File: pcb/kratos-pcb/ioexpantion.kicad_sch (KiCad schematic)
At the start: 3 parts, among them IC2 SN74HC595N, U3 ULN2803A

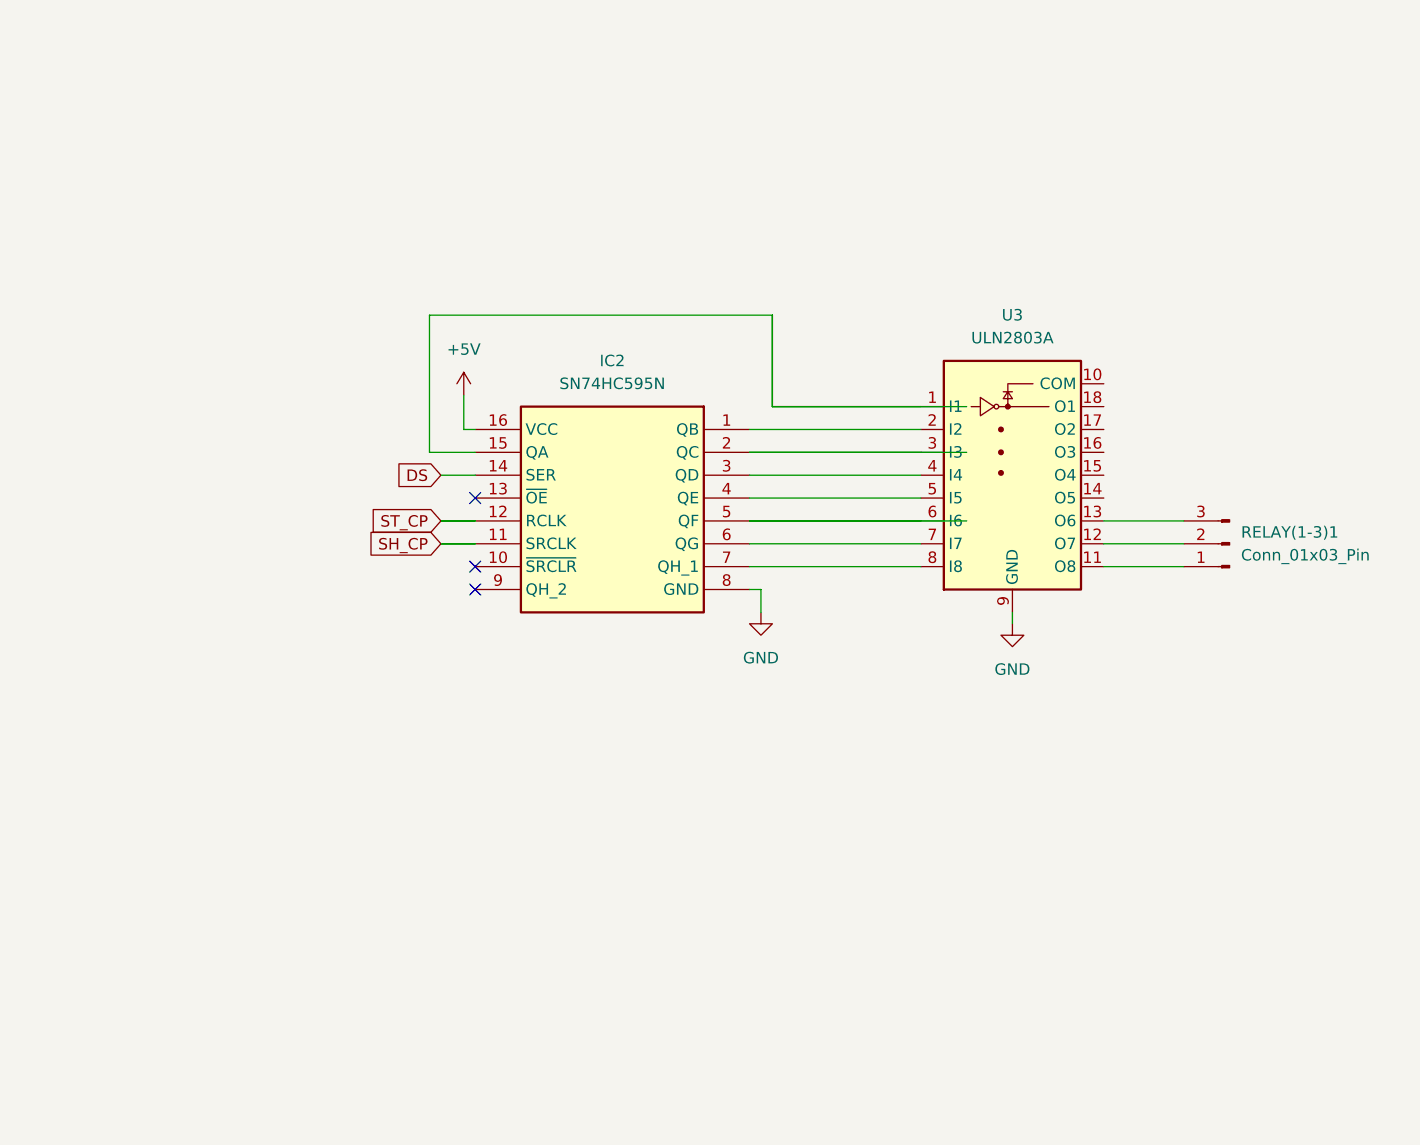
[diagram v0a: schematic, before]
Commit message: ### update     - kicad schematic
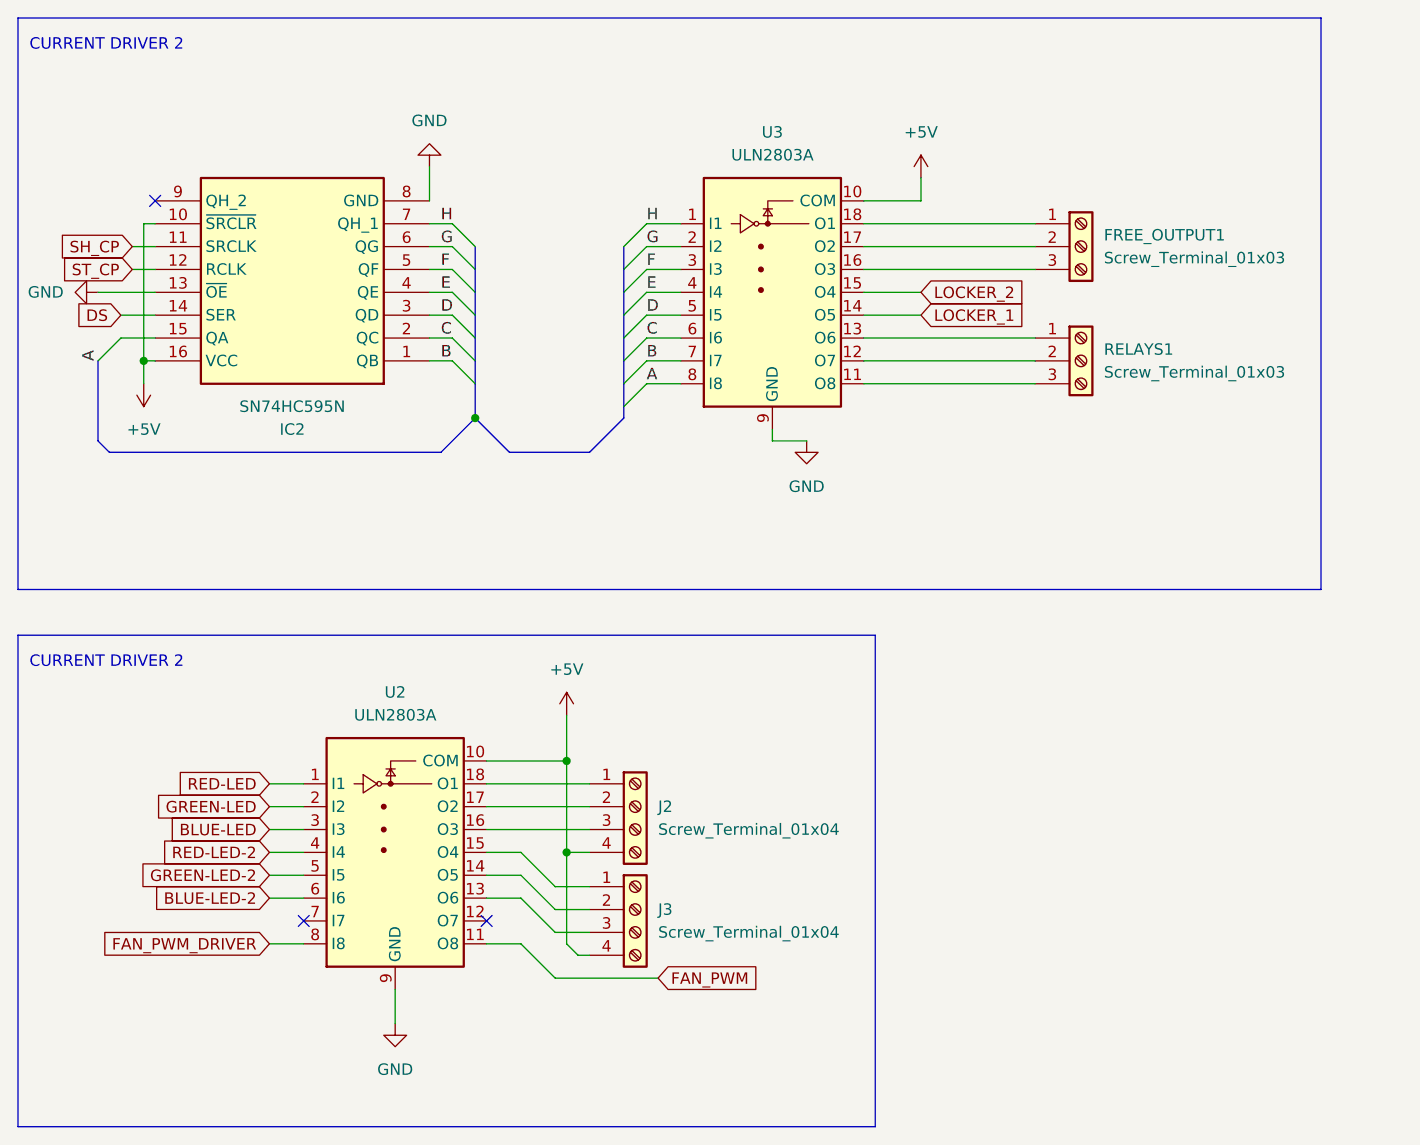
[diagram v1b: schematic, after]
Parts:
- removed RELAY(1-3)1: Conn_01x03_Pin, symbol Connector:Conn_01x03_Pin
- added FREE_OUTPUT1, RELAYS1: Screw_Terminal_01x03, TerminalBlock_4Ucon:TerminalBlock_4Ucon_1x03_P3.50mm_Horizontal, symbol Connector:Screw_Terminal_01x03
- added J2, J3: Screw_Terminal_01x04, TerminalBlock:TerminalBlock_bornier-4_P5.08mm, symbol Connector:Screw_Terminal_01x04
- added U2: ULN2803A, ULN2803A:ULN2803A, symbol Transistor_Array:ULN2803A
- IC2: footprint SN74HC595N:DIP794W53P254L1930H508Q16N -> DIP794W53P254L1930H508Q16N
- U3: footprint (none) -> ULN2803A:ULN2803A
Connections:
- net +5V: now also IC2.10 (~{SRCLR}), U3.10 (COM), J2.4 (Pin_4), J3.4 (Pin_4), U2.10 (COM)
- net GND: now also IC2.13 (~{OE}), U2.9 (GND)
- net B: now reaches IC2.1 (QB)
- net B: now also U3.7 (I7); no longer U3.2 (I2)
- net at IC2.15 (QA): no longer U3.1 (I1)
- net C: now reaches IC2.2 (QC)
- net C: now also U3.6 (I6); no longer U3.3 (I3)
- net D: now reaches IC2.3 (QD)
- net D: now also U3.5 (I5); no longer U3.4 (I4)
- net E: now reaches IC2.4 (QE)
- net E: now also U3.4 (I4); no longer U3.5 (I5)
- net F: now reaches IC2.5 (QF)
- net F: now also U3.3 (I3); no longer U3.6 (I6)
- net G: now reaches IC2.6 (QG)
- net G: now also U3.2 (I2); no longer U3.7 (I7)
- net A: now reaches U3.8 (I8)
- net A: no longer IC2.7 (QH_1)
- net at U3.11 (O8): now also RELAYS1.3 (Pin_3)
- net at U3.12 (O7): now also RELAYS1.2 (Pin_2)
- net at U3.13 (O6): now also RELAYS1.1 (Pin_1)
- net LOCKER_1: now reaches U3.14 (O5)
- net LOCKER_2: now reaches U3.15 (O4)
- net at U3.16 (O3): now also FREE_OUTPUT1.3 (Pin_3)
- net at U3.17 (O2): now also FREE_OUTPUT1.2 (Pin_2)
- net at U3.18 (O1): now also FREE_OUTPUT1.1 (Pin_1)
- new net: J3.3 (Pin_3), U2.13 (O6)
- new net: J3.2 (Pin_2), U2.14 (O5)
- new net: J3.1 (Pin_1), U2.15 (O4)
- new net: J2.3 (Pin_3), U2.16 (O3)
- new net: J2.2 (Pin_2), U2.17 (O2)
- new net: J2.1 (Pin_1), U2.18 (O1)
- new net BLUE-LED: U2.3 (I3)
- new net BLUE-LED-2: U2.6 (I6)
- new net FAN_PWM: U2.11 (O8)
- new net FAN_PWM_DRIVER: U2.8 (I8)
- new net GREEN-LED: U2.2 (I2)
- new net GREEN-LED-2: U2.5 (I5)
- new net H: IC2.7 (QH_1), U3.1 (I1)
- new net RED-LED: U2.1 (I1)
- new net RED-LED-2: U2.4 (I4)
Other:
- note added: "CURRENT DRIVER 2"
- moved on the sheet: IC2, U3
